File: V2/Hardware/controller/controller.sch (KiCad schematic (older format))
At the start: 45 parts, among them J0 Molex_PSU_F, J2 Flat_7seg_F, J3 Rpi_DATA_F_3.3V, Q0 BD139-16, Q1 BD139-16, Q2 BD139-16, Q3 BD139-16, Q4 BD139-16, Q5 BD139-16, Q6 BD139-16, U1 ATtiny2313-20PU

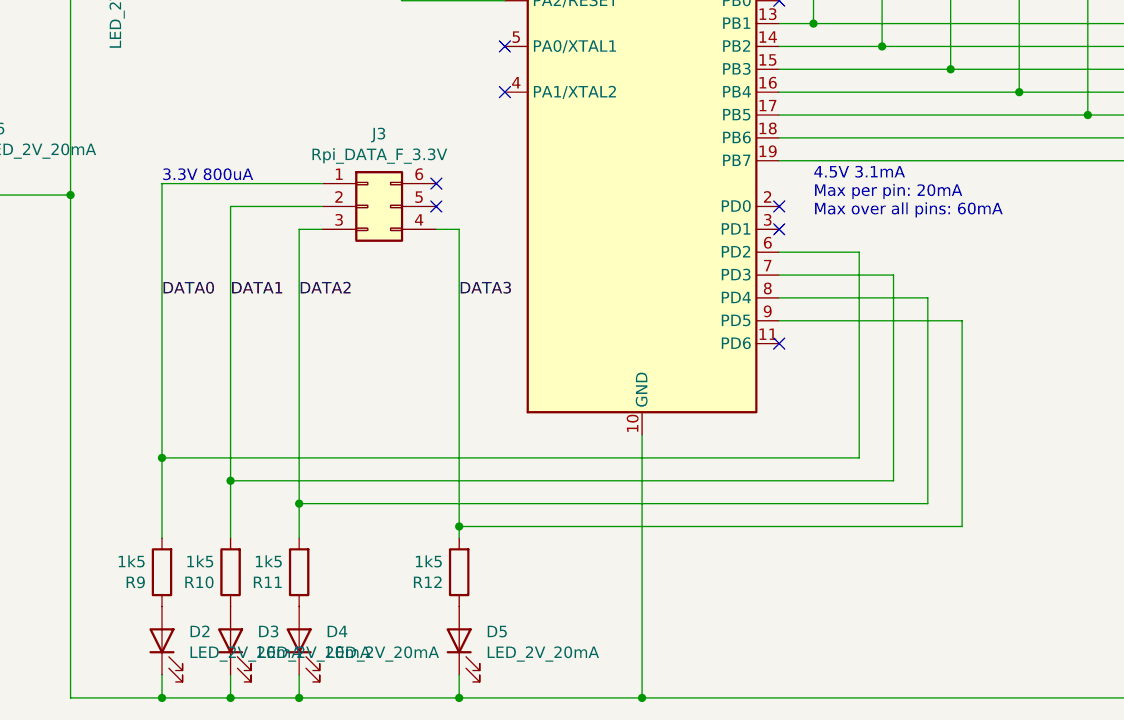
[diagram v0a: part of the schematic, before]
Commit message: Finish PCBs
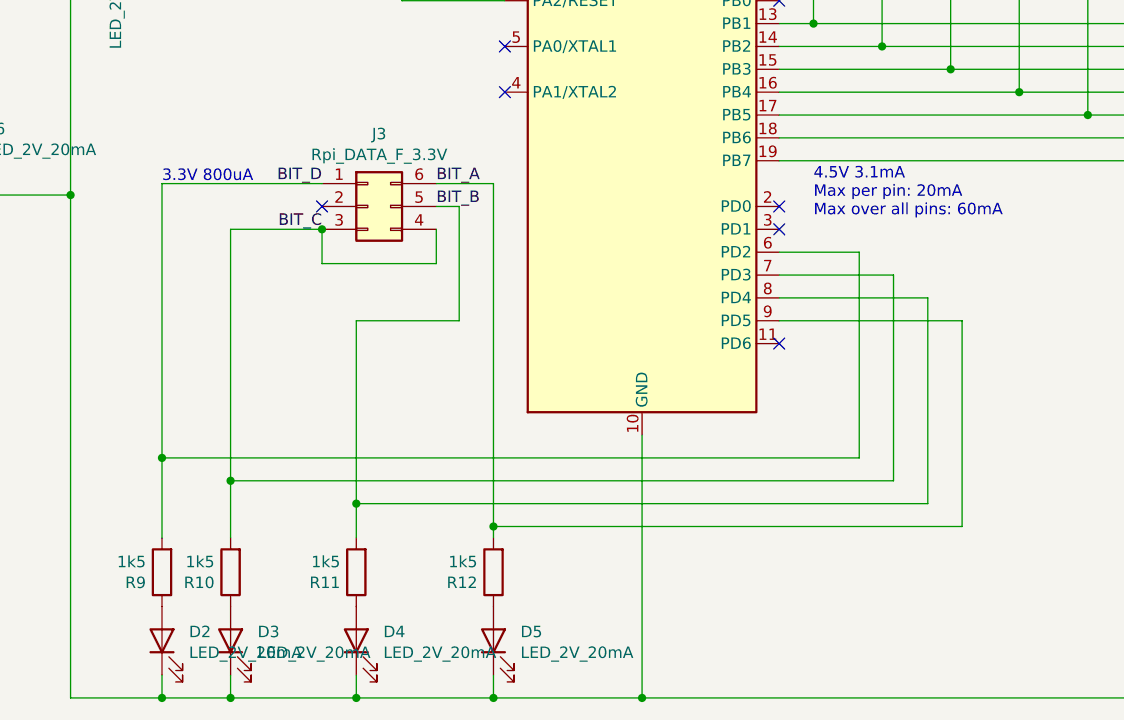
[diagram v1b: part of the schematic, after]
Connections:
- net BIT_B: now reaches J3.5 (Pin_5)
- net BIT_B: now also R11.2, U1.8 (PD4)
- net BIT_A: now reaches J3.6 (Pin_6)
- net BIT_A: now also R12.2, U1.9 (PD5)
- net DATA0 renamed BIT_D
- net DATA1 renamed BIT_C
- net BIT_C: now also J3.3 (Pin_3), J3.4 (Pin_4); no longer J3.2 (Pin_2)
- removed net DATA2: J3.3 (Pin_3), R11.2, U1.8 (PD4)
- removed net DATA3: J3.4 (Pin_4), R12.2, U1.9 (PD5)
- no-connect marks 8 -> 7
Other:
- moved on the sheet: D4, D5, R11, R12
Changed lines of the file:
@@
 L Device:R R12
 U 1 1 5EB47108
-P 3700 4350
-F 0 "R12" H 3770 4396 50  0000 L CNN
-F 1 "1k5" H 3770 4305 50  0000 L CNN
-F 2 "Resistor_THT:R_Axial_DIN0207_L6.3mm_D2.5mm_P10.16mm_Horizontal" V 3630 4350 50  0001 C CNN
-F 3 "~" H 3700 4350 50  0001 C CNN
-	1    3700 4350
+P 3850 4350
+F 0 "R12" H 3920 4396 50  0000 L CNN
+F 1 "1k5" H 3920 4305 50  0000 L CNN
+F 2 "Resistor_THT:R_Axial_DIN0207_L6.3mm_D2.5mm_P10.16mm_Horizontal" V 3780 4350 50  0001 C CNN
+F 3 "~" H 3850 4350 50  0001 C CNN
+	1    3850 4350
 	-1   0    0    1
 $EndComp
@@
 Wire Wire Line
 	2400 1450 2550 1450
-NoConn ~ 3600 2650
-Text Label 2700 3150 0    50   ~ 0
-DATA1
-Text Label 3000 3150 0    50   ~ 0
-DATA2
-Text Label 3700 3150 0    50   ~ 0
-DATA3
+Text Label 3600 2750 0    50   ~ 0
+BIT_B
 $Comp
 L Connector_Generic:Conn_01x04 J0
@@
 $EndComp
 $Comp
-L Connector_Generic:Conn_02x03_Counter_Clockwise J3
-U 1 1 5EA33B7C
-P 3300 2750
-F 0 "J3" H 3350 3067 50  0000 C CNN
-F 1 "Rpi_DATA_F_3.3V" H 3350 2976 50  0000 C CNN
-F 2 "Connector_PinHeader_2.54mm:PinHeader_2x03_P2.54mm_Horizontal" H 3300 2750 50  0001 C CNN
-F 3 "~" H 3300 2750 50  0001 C CNN
-	1    3300 2750
-	1    0    0    -1
-$EndComp
-$Comp
 L Connector_Generic:Conn_02x04_Counter_Clockwise J2
 U 1 1 5EACC56A
@@
 	1    0    0    -1
 $EndComp
-Wire Wire Line
-	3100 2850 3000 2850
-Wire Wire Line
-	3700 2850 3600 2850
 $Comp
 L power:PWR_FLAG #FLG0101
@@
 	1    0    0    -1
 $EndComp
-NoConn ~ 3600 2750
 Wire Wire Line
 	1900 1250 4500 1250
@@
 L Device:R R11
 U 1 1 5EB45F1E
-P 3000 4350
-F 0 "R11" H 3070 4396 50  0000 L CNN
-F 1 "1k5" H 3070 4305 50  0000 L CNN
-F 2 "Resistor_THT:R_Axial_DIN0207_L6.3mm_D2.5mm_P10.16mm_Horizontal" V 2930 4350 50  0001 C CNN
-F 3 "~" H 3000 4350 50  0001 C CNN
-	1    3000 4350
+P 3250 4350
+F 0 "R11" H 3320 4396 50  0000 L CNN
+F 1 "1k5" H 3320 4305 50  0000 L CNN
+F 2 "Resistor_THT:R_Axial_DIN0207_L6.3mm_D2.5mm_P10.16mm_Horizontal" V 3180 4350 50  0001 C CNN
+F 3 "~" H 3250 4350 50  0001 C CNN
+	1    3250 4350
 	-1   0    0    1
 $EndComp
@@
 L Device:LED D4
 U 1 1 5FC9598B
-P 3000 4650
-F 0 "D4" V 3039 4532 50  0000 R CNN
-F 1 "LED_2V_20mA" V 2948 4532 50  0000 R CNN
-F 2 "LED_THT:LED_D5.0mm" H 3000 4650 50  0001 C CNN
-F 3 "~" H 3000 4650 50  0001 C CNN
-	1    3000 4650
+P 3250 4650
+F 0 "D4" V 3289 4532 50  0000 R CNN
+F 1 "LED_2V_20mA" V 3198 4532 50  0000 R CNN
+F 2 "LED_THT:LED_D5.0mm" H 3250 4650 50  0001 C CNN
+F 3 "~" H 3250 4650 50  0001 C CNN
+	1    3250 4650
 	0    -1   -1   0
 $EndComp
@@
 L Device:LED D5
 U 1 1 5FC961FF
-P 3700 4650
-F 0 "D5" V 3739 4532 50  0000 R CNN
-F 1 "LED_2V_20mA" V 3648 4532 50  0000 R CNN
-F 2 "LED_THT:LED_D5.0mm" H 3700 4650 50  0001 C CNN
-F 3 "~" H 3700 4650 50  0001 C CNN
-	1    3700 4650
+P 3850 4650
+F 0 "D5" V 3889 4532 50  0000 R CNN
+F 1 "LED_2V_20mA" V 3798 4532 50  0000 R CNN
+F 2 "LED_THT:LED_D5.0mm" H 3850 4650 50  0001 C CNN
+F 3 "~" H 3850 4650 50  0001 C CNN
+	1    3850 4650
 	0    -1   -1   0
 $EndComp
@@
 	0    -1   -1   0
 $EndComp
-Text Label 2400 3150 0    50   ~ 0
-DATA0
 $Comp
 L Device:R R9
@@
 	2000 4900 2400 4900
 Wire Wire Line
-	3000 2850 3000 4050
-Wire Wire Line
-	2700 2750 2700 3950
-Wire Wire Line
-	2700 2750 3100 2750
-Wire Wire Line
-	2400 2650 2400 3850
-Wire Wire Line
-	2400 2650 3100 2650
-Wire Wire Line
 	2400 4800 2400 4900
 Connection ~ 2400 4900
@@
 Connection ~ 2700 4900
 Wire Wire Line
-	2700 4900 3000 4900
-Wire Wire Line
-	3000 4800 3000 4900
-Connection ~ 3000 4900
-Wire Wire Line
-	3000 4900 3700 4900
-Wire Wire Line
-	3700 4800 3700 4900
-Connection ~ 3700 4900
-Wire Wire Line
-	3700 4900 4500 4900
+	2700 4900 3250 4900
+Wire Wire Line
+	3250 4800 3250 4900
+Connection ~ 3250 4900
+Wire Wire Line
+	3250 4900 3850 4900
+Wire Wire Line
+	3850 4800 3850 4900
+Connection ~ 3850 4900
 Wire Wire Line
 	2400 3850 5450 3850
@@
 	2700 3950 2700 4200
 Wire Wire Line
-	3000 4050 5750 4050
-Connection ~ 3000 4050
-Wire Wire Line
-	3000 4050 3000 4200
-Wire Wire Line
-	3700 2850 3700 4150
-Wire Wire Line
-	3700 4150 5900 4150
-Connection ~ 3700 4150
-Wire Wire Line
-	3700 4150 3700 4200
+	3250 4050 5750 4050
+Wire Wire Line
+	3250 4050 3250 4200
 Wire Wire Line
 	5450 2950 5100 2950
@@
 Wire Wire Line
 	9800 1700 9800 4350
+Wire Wire Line
+	2700 2850 2700 3950
+Wire Wire Line
+	3700 2750 3600 2750
+Text Label 3100 2650 2    50   ~ 0
+BIT_D
+Text Label 3100 2850 2    50   ~ 0
+BIT_C
+Text Label 3600 2650 0    50   ~ 0
+BIT_A
+$Comp
+L Connector_Generic:Conn_02x03_Counter_Clockwise J3
+U 1 1 5EA33B7C
+P 3300 2750
+F 0 "J3" H 3350 3067 50  0000 C CNN
+F 1 "Rpi_DATA_F_3.3V" H 3350 2976 50  0000 C CNN
+F 2 "Connector_PinHeader_2.54mm:PinHeader_2x03_P2.54mm_Horizontal" H 3300 2750 50  0001 C CNN
+F 3 "~" H 3300 2750 50  0001 C CNN
+	1    3300 2750
+	1    0    0    -1
+$EndComp
+Wire Wire Line
+	3850 4150 5900 4150
+Wire Wire Line
+	3850 4150 3850 4200
+Connection ~ 3850 4150
+Wire Wire Line
+	3850 4900 4500 4900
+Wire Wire Line
+	3850 2650 3600 2650
+Wire Wire Line
+	3850 2650 3850 4150
+NoConn ~ 3100 2750
+Wire Wire Line
+	2700 2850 3100 2850
+Wire Wire Line
+	2400 2650 3100 2650
+Wire Wire Line
+	2400 2650 2400 3850
+Wire Wire Line
+	3700 2750 3700 3250
+Wire Wire Line
+	3700 3250 3250 3250
+Wire Wire Line
+	3250 3250 3250 4050
+Connection ~ 3250 4050
+Wire Wire Line
+	3100 2850 3100 3000
+Wire Wire Line
+	3100 3000 3600 3000
+Wire Wire Line
+	3600 3000 3600 2850
+Connection ~ 3100 2850
 $EndSCHEMATC
